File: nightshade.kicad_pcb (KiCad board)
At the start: 4 copper layers, 187.3 x 76.2 mm, 101 parts, among them J1 Bus_ISA_16bit, J2 DE15_Plug_HighDensity_Mountin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, J3 Conn_02x13_Odd_Even, Q1 MMBT3904, U1 GD542x_ISA, U10 74HCT244, U11 SOJ_256Kx16, U12 SOJ_256Kx16, U2 SOJ_256Kx16, U3 SOJ_256Kx16, U4 TL431DBZ, U5 93CxxA, U6 27C256, U7 LF50_TO252, U8 74HCT244, U9 27C256, Y1 14.31818MHz

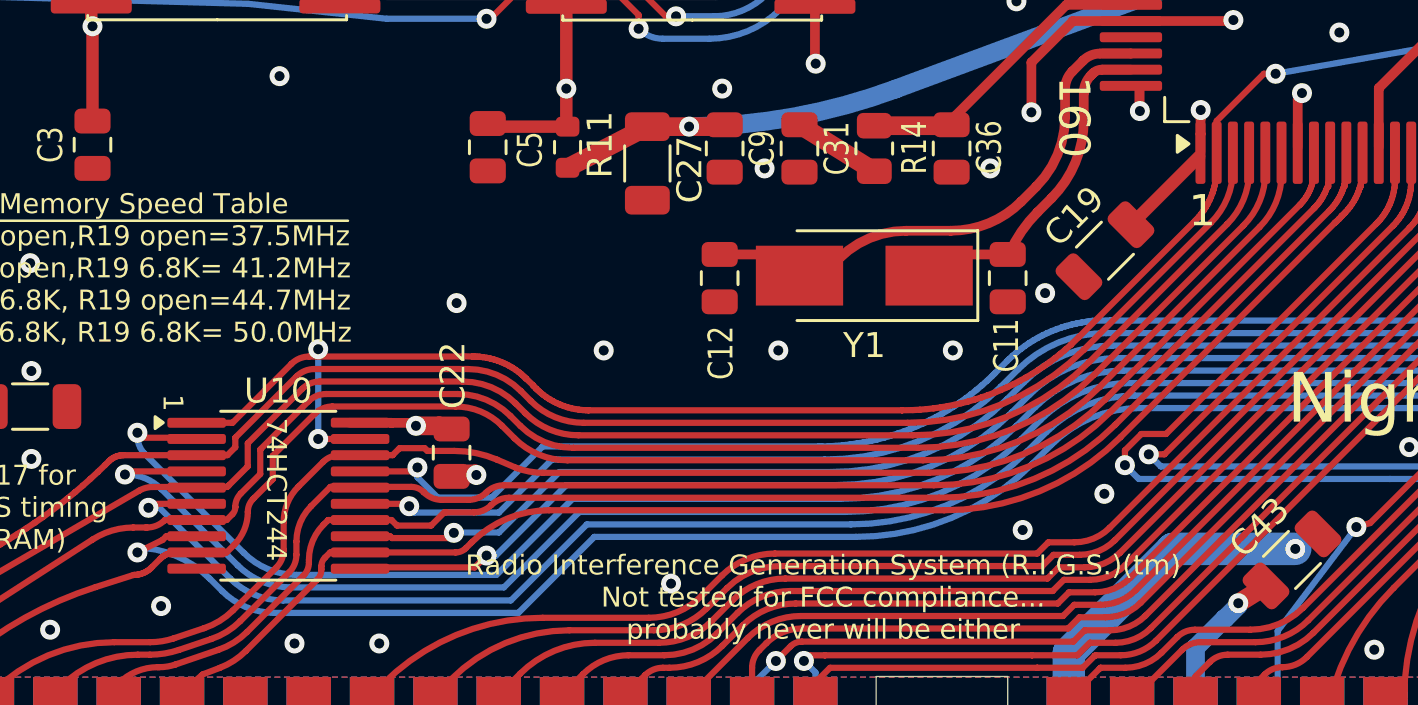
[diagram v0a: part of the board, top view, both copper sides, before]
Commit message: Add files via upload
More minor fixes.
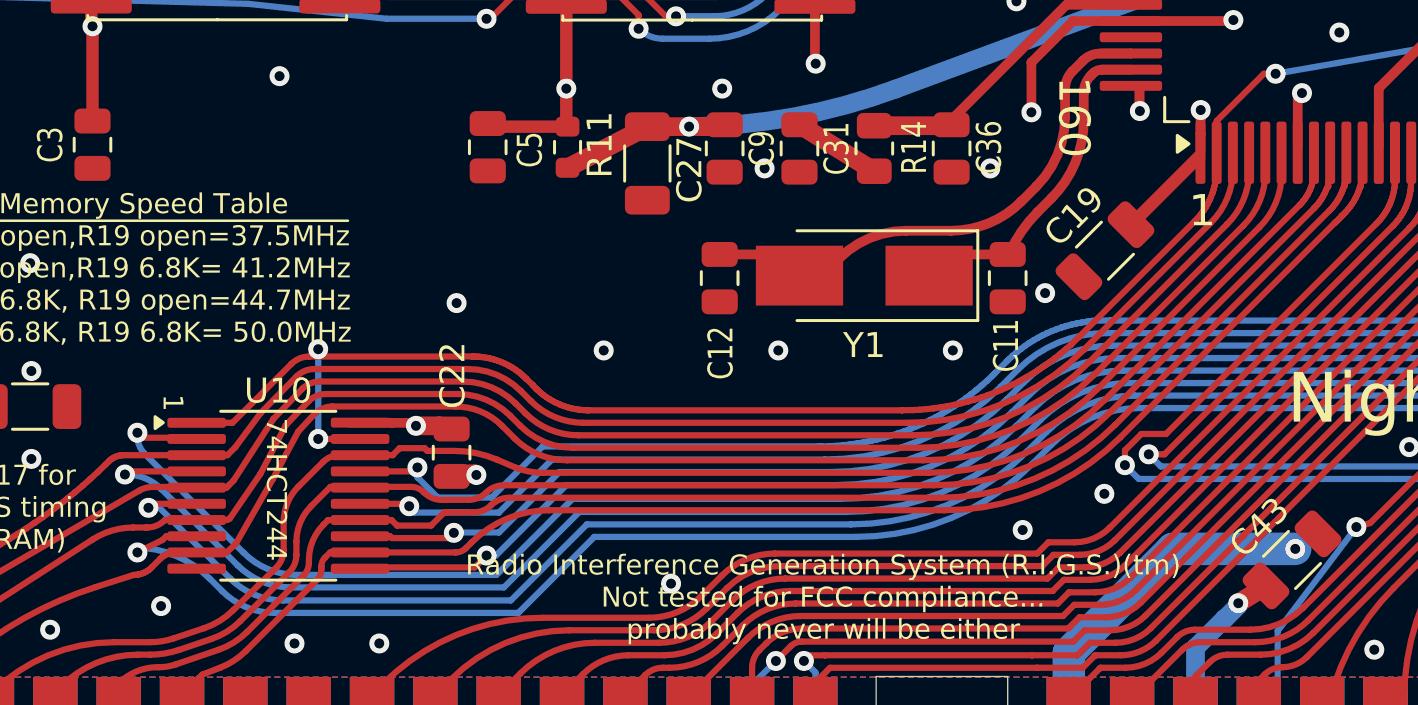
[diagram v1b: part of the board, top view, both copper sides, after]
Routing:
- net GND: track 345.9 -> 344.8 mm
